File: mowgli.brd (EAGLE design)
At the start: 71.1 x 22.9 mm, 19 parts, among them IC1 ATMEGA, IC2 MCP1702-33, X1 16 MHz, X2 uFL, X3 JSTPH

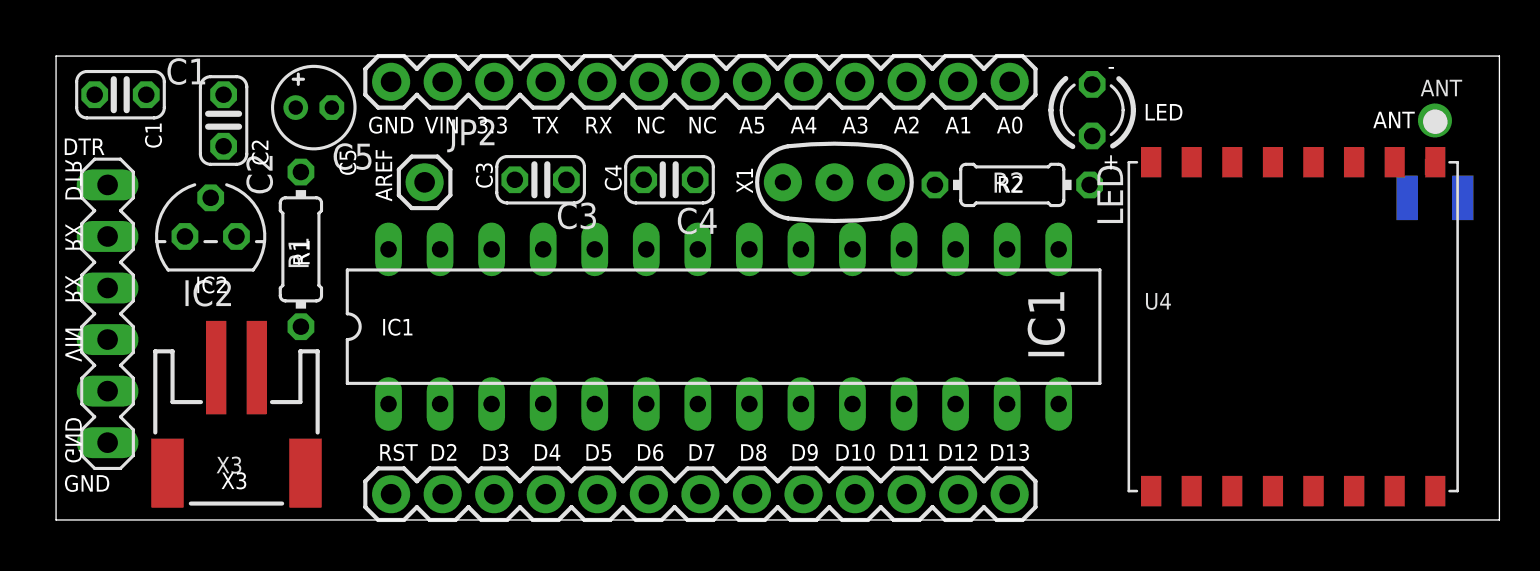
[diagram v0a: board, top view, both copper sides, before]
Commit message: update
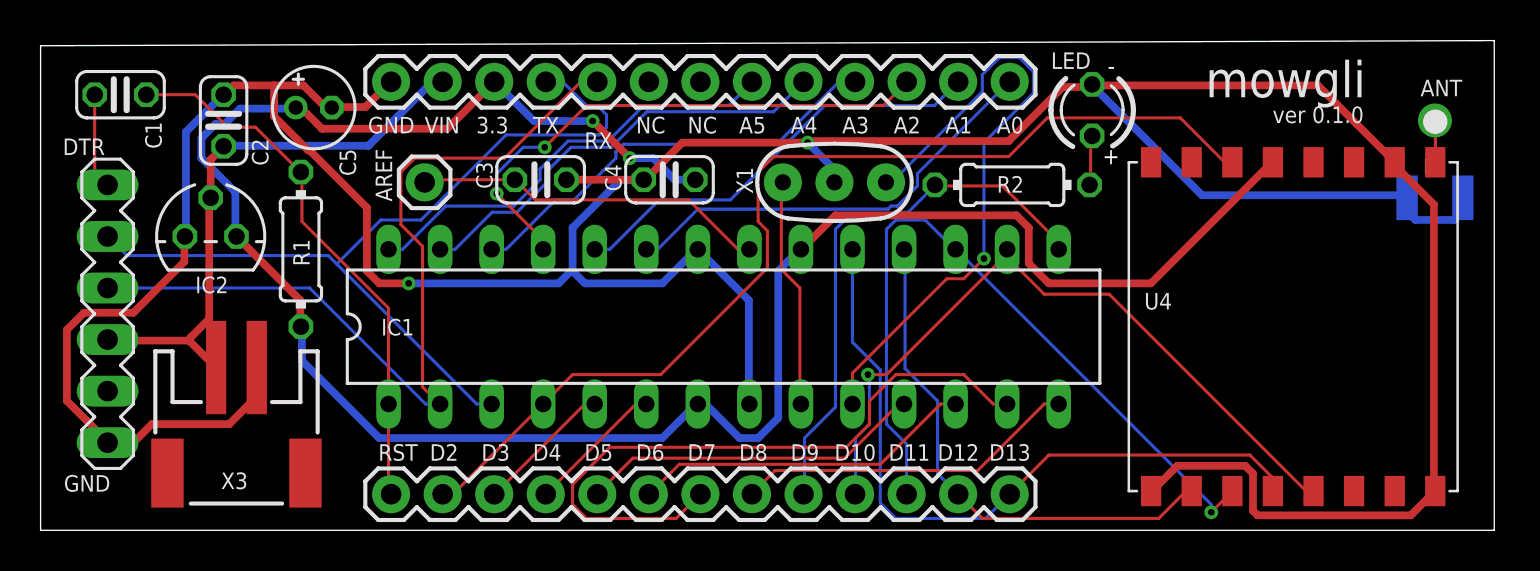
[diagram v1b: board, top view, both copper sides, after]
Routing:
- net GND: track 0.00 -> 189.1 mm, vias 0 -> 2
- net VCC: track 0.00 -> 105.9 mm, vias 0 -> 2
- net D2: track 0.00 -> 50.9 mm
- net D1_TX: track 0.00 -> 42.7 mm
- net D0_RX: track 0.00 -> 42.5 mm
- net D11_MOSI: track 0.00 -> 37.3 mm, vias 0 -> 1
- net D10_SS: track 0.00 -> 36.2 mm, vias 0 -> 1
- net D13_SCK: track 0.00 -> 35.2 mm
- net D7: track 0.00 -> 33.0 mm
- net N$21: track 0.00 -> 31.2 mm, vias 0 -> 1
- net PWR: track 0.00 -> 28.3 mm
- net D9: track 0.00 -> 27.2 mm
- net RST: track 0.00 -> 27.0 mm
- net A2: track 0.00 -> 26.8 mm, vias 0 -> 2
- net D12_MISO: track 0.00 -> 25.8 mm
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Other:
- board size 71.1 x 22.9 mm -> 71.6 x 24.1 mm
- board text added: "https://github.com/p-v-o-s/mowgli"
- board text added: "mowgli"
- board text added: "ver 0.1.0"
- board text removed: "ANT"
